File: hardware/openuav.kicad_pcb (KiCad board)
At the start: 4 copper layers, 36 x 36 mm, 92 parts, among them J1 Conn_01x01, J10 Conn_01x01, J11 Conn_01x01, J12 Conn_01x01, J13 Conn_01x01, J14 Conn_01x01, J15 Conn_01x01, J16 Conn_01x01, J17 Conn_01x01, J18 Conn_01x01, J19 Conn_01x01, J2 Conn_01x01, J20 Conn_01x01, J21 Conn_01x01, J22 Conn_01x01, J23 Conn_01x01, J24 Conn_01x01, J25 Conn_01x01, J3 Conn_01x01, J4 Conn_01x01, J5 Conn_01x01, J6 Conn_01x01, J7 Conn_01x01, J8 Conn_01x01, J9 Conn_01x01, J99 USB_C_Receptacle_USB2.0, SW1 SW_Push, SW2 SW_Push, U1 STM32G431CBUx, U2 LPS22HH, U3 LSM6DSR, U6 W25N01GVZEIG, U7 TLV75733PDBV

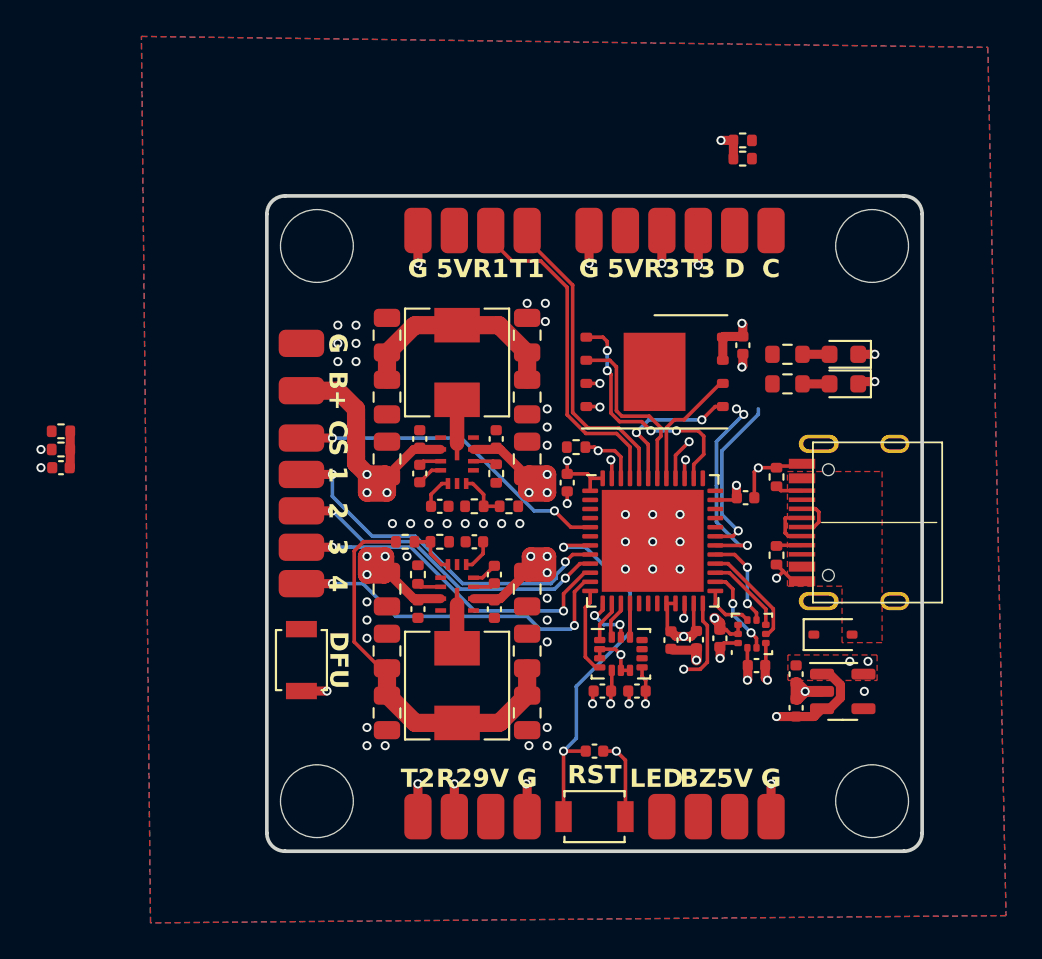
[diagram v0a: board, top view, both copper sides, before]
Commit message: Work in progress new SMPS
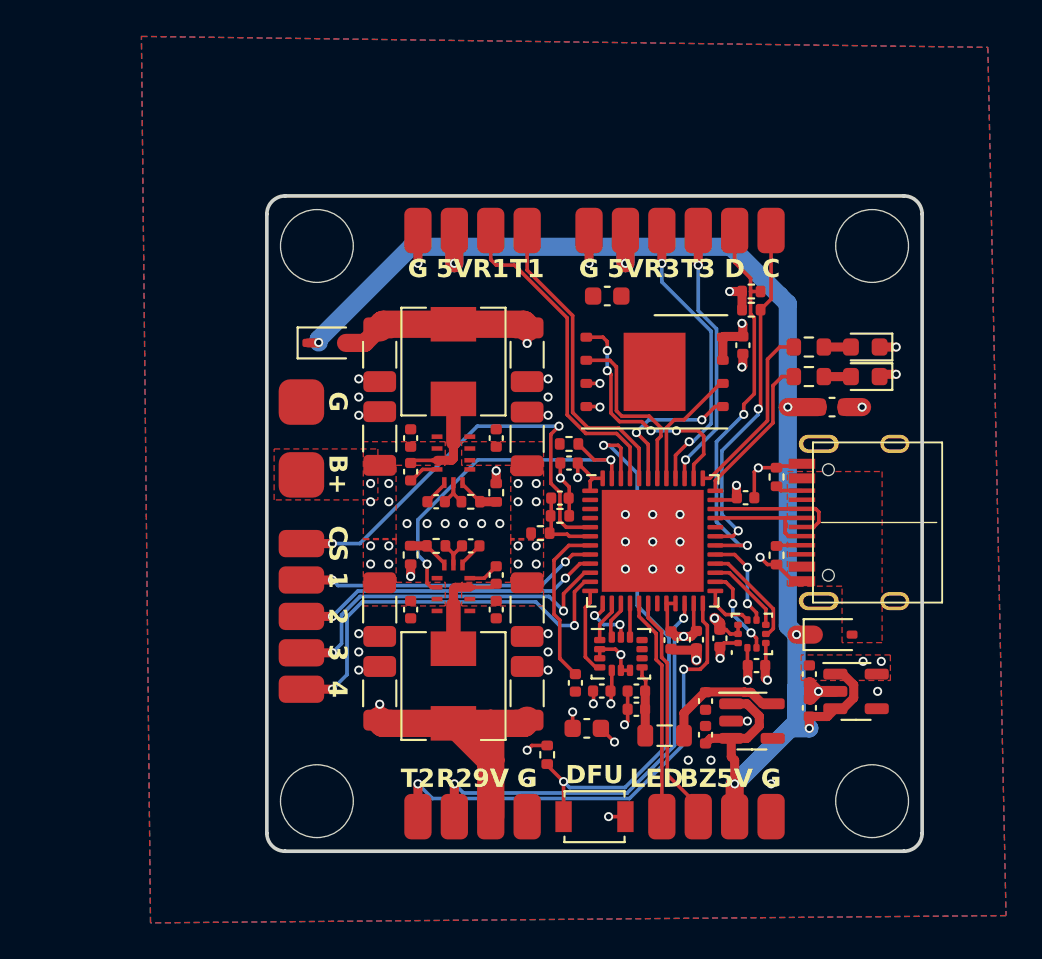
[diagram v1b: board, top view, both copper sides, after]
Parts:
- removed the C10 at (144.3, 61.0)
- removed the C15 at (136.6, 61.0)
- removed the C17 at (144.3, 64.5)
- removed the C18 at (136.6, 64.5)
- removed the C19 at (142.6, 63.4)
- removed the C2 at (139.5, 67.0)
- removed the C20 at (136.6, 57.6)
- removed the C20 at (144.3, 78.4)
- removed the C21 at (138.4, 63.4)
- removed the C22 at (144.3, 57.6)
- removed the C22 at (136.6, 78.4)
- removed the C9 at (138.4, 65.2)
- removed the L1 at (140.4, 59.1)
- removed the R3 at (141.4, 67.0)
- removed the R4 at (143.3, 67.0)
- removed R5 (x2): 10k, Resistor_SMD:R_0402_1005Metric
- removed SW2: SW_Push, Button_Switch_SMD:SW_SPST_B3U-1000P
- removed the U4 at (140.4, 64.4)
- added C20: 10u, Capacitor_SMD:C_1206_3216Metric, F.Cu at (144.3, 63.4)
- added C22: 100n, Capacitor_SMD:C_0402_1005Metric, F.Cu at (142.6, 63.3)
- added C23: 10u, Capacitor_SMD:C_1206_3216Metric, F.Cu at (136.2, 63.3)
- added C26: 1u, Capacitor_SMD:C_0402_1005Metric, F.Cu at (139.3, 66.8)
- added C27: 100n, Capacitor_SMD:C_0402_1005Metric, F.Cu at (137.9, 65.2)
- added C28: 22u, Capacitor_SMD:C_1206_3216Metric, F.Cu at (144.3, 58.7)
- added C29: 22u, Capacitor_SMD:C_1206_3216Metric, F.Cu at (136.2, 58.7)
- added C30: 1u, Capacitor_SMD:C_0402_1005Metric, F.Cu at (150.3, 78.2)
- added C31: 1u, Capacitor_SMD:C_0402_1005Metric, F.Cu at (154.1, 79.6)
- added C32: 1u, Capacitor_SMD:C_0402_1005Metric, F.Cu at (154.1, 77.8)
- added C33: 10u, Capacitor_SMD:C_0603_1608Metric, F.Cu at (148.7, 55.5)
- added C34: 10u, Capacitor_SMD:C_0603_1608Metric, F.Cu at (147.6, 79.2)
- added C35: 10u, Capacitor_SMD:C_0603_1608Metric, F.Cu at (161.1, 61.6)
- added C8: 100n, Capacitor_SMD:C_0402_1005Metric, F.Cu at (137.9, 63.3)
- added D4: PMEG2020AEA, Diode_SMD:D_SOD-323, F.Cu at (133.3, 58.1)
- added FB1: FerriteBead, Inductor_SMD:L_0805_2012Metric, F.Cu at (151.8, 79.7)
- added L2: 10u, Inductor_SMD:L_Sunlord_MWSA0503S, F.Cu at (140.2, 59.1)
- added R13: 10k, Resistor_SMD:R_0402_1005Metric, F.Cu at (146.6, 63.6)
- added R14: 22k, Resistor_SMD:R_0402_1005Metric, F.Cu at (142.6, 66.3)
- added R15: 2.44k, Resistor_SMD:R_0402_1005Metric, F.Cu at (141.2, 66.8)
- added U5: ~, footprints:RNX0012B, F.Cu at (140.2, 64.3)
- added U8: TLV75733PDBV, Package_TO_SOT_SMD:SOT-23-5, F.Cu at (156.7, 78.8)
- C10, C15, C17, C18: footprint Capacitor_SMD:C_0805_2012Metric -> Capacitor_SMD:C_1206_3216Metric
- J15, J16: footprint footprints:smallpad -> footprints:largepad
- L1: value 6.8u -> 10u
- moved R6 27.7 mm to (146.1, 67.6), turned to 0 degrees
- moved C14 27.5 mm to (146.1, 66.6), turned to 0 degrees
- moved R12 26.9 mm to (145.0, 68.5)
- moved SW1 18.3 mm to (148.0, 84.1), turned to 180 degrees
- moved R8 17.0 mm to (145.4, 80.7), turned to 90 degrees
- moved R10 8.31 mm to (156.6, 56.2)
- moved R9 8.31 mm to (156.6, 55.2)
- moved J18 5.80 mm to (131.9, 69.1)
- moved J22 5.80 mm to (131.9, 71.1)
- moved J23 5.80 mm to (131.9, 73.1)
- moved J24 5.80 mm to (131.9, 75.1)
- moved J25 5.80 mm to (131.9, 77.1)
- moved J15 4.62 mm to (131.9, 65.3)
- moved C1 3.89 mm to (146.9, 76.8), turned to 90 degrees
- moved J16 3.23 mm to (131.9, 61.3)
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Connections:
- C10 pad 1: Net-(C10-Pad1) -> +9V
- C15 pad 1: Net-(C10-Pad1) -> +9V
- C3 pad 1: +3V3 -> VDDA
- L1 pad 2: Net-(C10-Pad1) -> +9V
- R4 pad 1: Net-(C10-Pad1) -> +9V
- U3 pad 8: +3V3 -> VDDA
- U4 pad 9: 10VEN -> 9VEN
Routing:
- net +5V: track 5.91 -> 89.5 mm, vias 1 -> 7
- net +BATT: track 37.6 -> 0.00 mm, vias 12 -> 16
- net Net-(C10-Pad1): track 33.8 -> 0.00 mm
- net BOOT0: track 3.35 -> 30.8 mm, vias 1 -> 2
- net +9V: track 0.00 -> 25.5 mm, vias 0 -> 2
- net UART_4_RX: track 2.63 -> 23.2 mm
- net UART_4_TX: track 6.59 -> 26.9 mm
- net Net-(D4-A): track 0.00 -> 19.7 mm, vias 0 -> 2
- net 9VEN: track 1.03 -> 19.5 mm, vias 1 -> 2
- net PWM_6: track 0.00 -> 12.9 mm
- net PWM_5: track 0.00 -> 12.2 mm
- net NRST: track 21.3 -> 9.07 mm, vias 2 -> 0
- net UART_3_TX: track 2.93 -> 14.8 mm
- net UART_3_RX: track 4.12 -> 15.7 mm
- net I2C_SDA: track 10.5 -> 21.9 mm
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- added copper zone on F.Cu, net +BATT
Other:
- board text removed: "RST"
